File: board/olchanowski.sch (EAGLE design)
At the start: 196 parts, among them IC1 LPC1768, J1 B4B-XH-A(LF)(SN), J10 B4B-XH-A(LF)(SN), J2 B4B-XH-A(LF)(SN), J3 B4B-XH-A(LF)(SN), J4 ARJM11D7-009-AB-ER2-T, J5 B4B-XH-A(LF)(SN), J6 USB-C-FEMALE, J7 1744428-4, J8 282814-4, J9 1-281742-2, P1 TPSM53602, Q10 SSM3K329R,LF, Q11 SSM3K329R,LF, Q3 SIJA58DP, Q4 SIJA58DP, Q5 SSM3K329R,LF, Q6 SSM3K329R,LF, Q7 SSM3K329R,LF, Q8 SSM3K329R,LF, Q9 PFETSM, SW1 SPST-2-4PIN, SW2 SPST-2-4PIN, U1 TMC2209-LA, U2 TMC2209-LA, U3 TMC2209-LA, U4 TMC2209-LA, U5 LAN8720, U6 74HC1G04, U7 LM5111, U8 NCP5661-0, U9 PCA9306DCTR, X1 X-AXIS, X2 X-AXIS, X3 X-AXIS, X4 FAN, X5 UI, X6 HB THERM, X7 SENSER

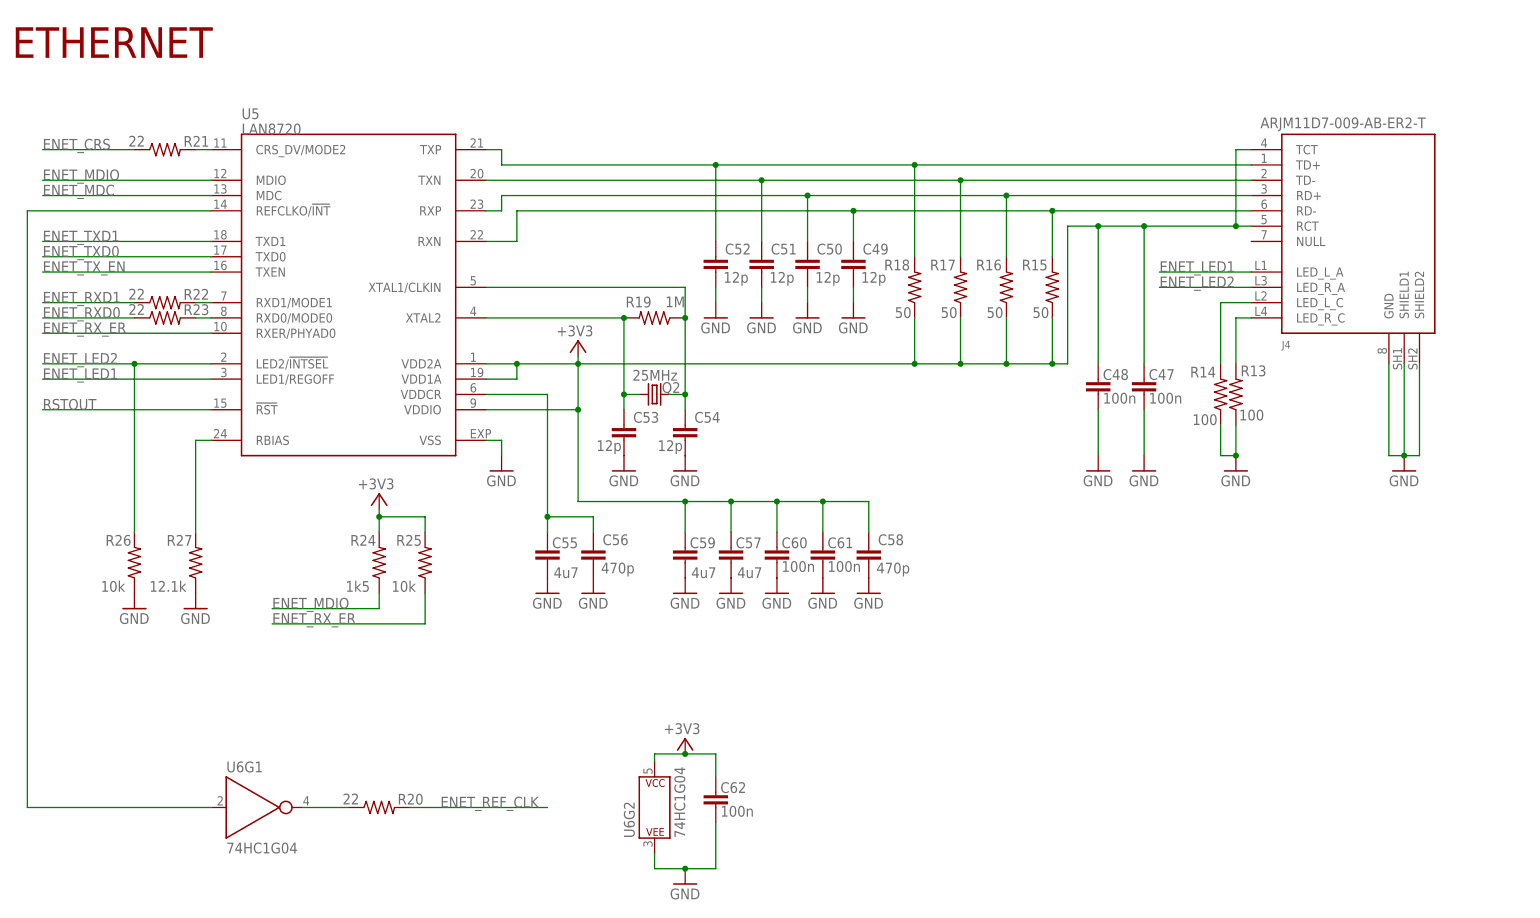
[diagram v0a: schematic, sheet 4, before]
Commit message: Started on board
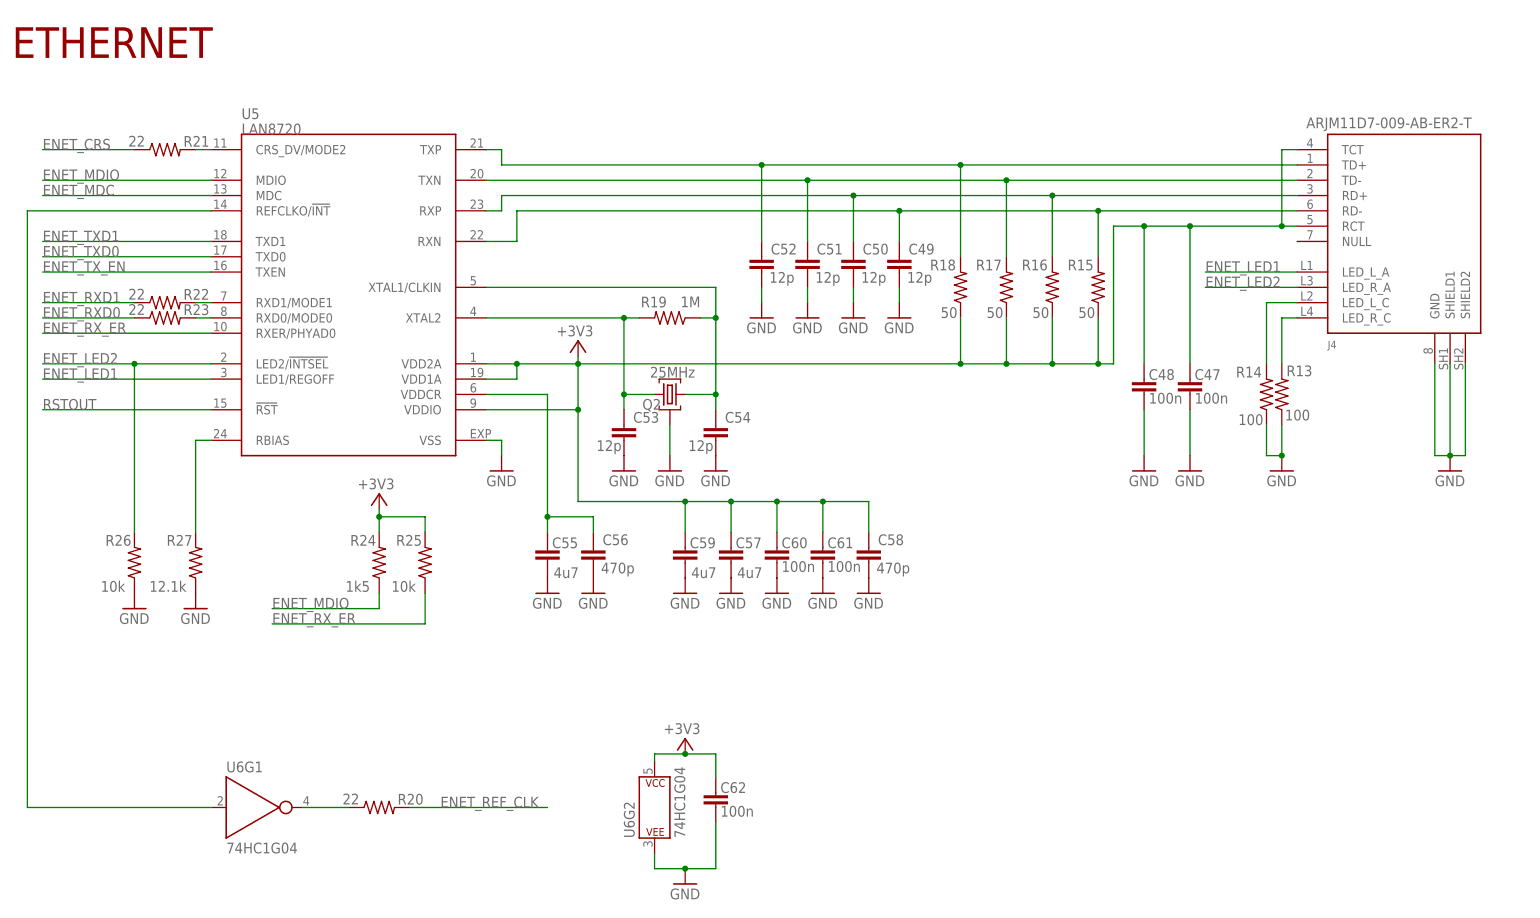
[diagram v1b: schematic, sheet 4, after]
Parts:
- added MNT1, MNT2, MNT3, MNT4, MNT5: MOUNT, robbe:MOUNT
- J1: value B4B-XH-A(LF)(SN) -> X-AXIS
- J2: value B4B-XH-A(LF)(SN) -> Y-AXIS
- J3: value B4B-XH-A(LF)(SN) -> Z_AXIS
- J5: value B4B-XH-A(LF)(SN) -> RGB LED
- Q1: value (none) -> 12MHz; device crystal:CRYSTALHC49UP -> robbe:CRYSTAL; FREQ 12MHz -> (none); MPN J49SMH-A-G-G-K-12M0 -> CX3225SB12000H0PSTC1
- Q2: value (none) -> 25MHz; device crystal:CRYSTALHC49UP -> robbe:CRYSTAL; FREQ 25MHz -> (none); MPN J49SMH-A-G-G-K-12M0 -> CX3225SB25000H0FLJCC
- X2: value X-AXIS -> Y-AXIS
- X3: value X-AXIS -> Z-AXIS
- X5: value UI -> LCD
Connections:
- removed net N$47: C53.1, Q2.2, R19.2, U5.XTAL2
- new net N$67: C53.1, Q2.1, R19.2, U5.XTAL2
- net GND: now also MNT1.MNT, MNT2.MNT, MNT3.MNT, MNT4.MNT, MNT5.MNT, Q1.2, Q2.2
- net N$1: now also Q1.1; no longer Q1.2
- net N$2: now also Q1.3; no longer Q1.1
- net N$48: now also Q2.3; no longer Q2.1
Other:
- note added: "MOUNTING"
- moved on the sheet: C2, C47, C48, C49, C50, C51, C52, C54, C85, C86, J4, R13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
